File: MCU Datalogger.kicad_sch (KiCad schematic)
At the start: 25 parts, among them U1 24LC1025, U2 DS1337S_, U3 24LC1025, U4 ATMEGA328P-AU, Y1 32.768 KHz, Y2 16 MHz

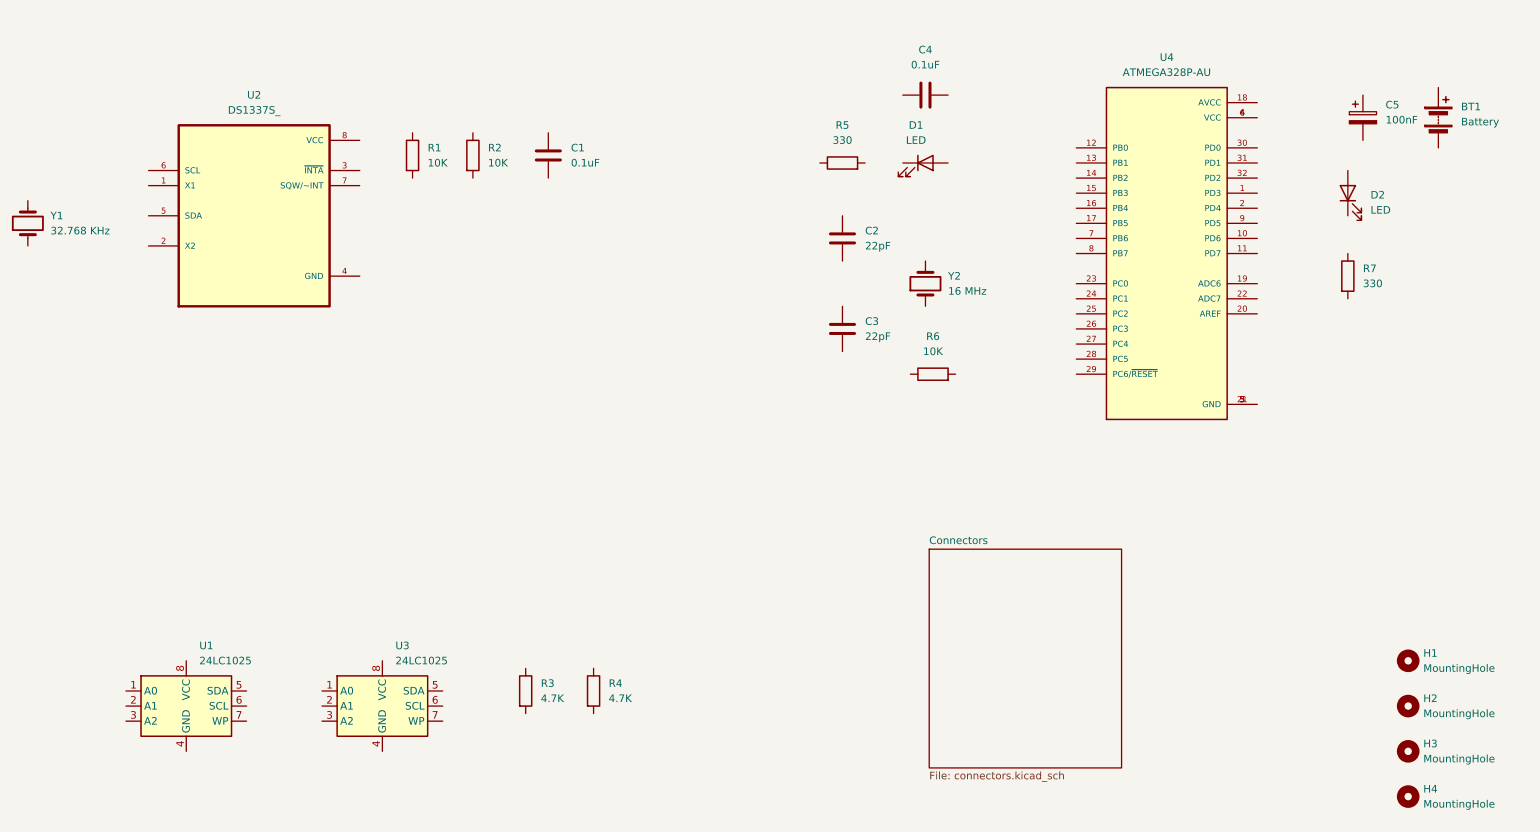
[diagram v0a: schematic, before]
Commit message: Test.
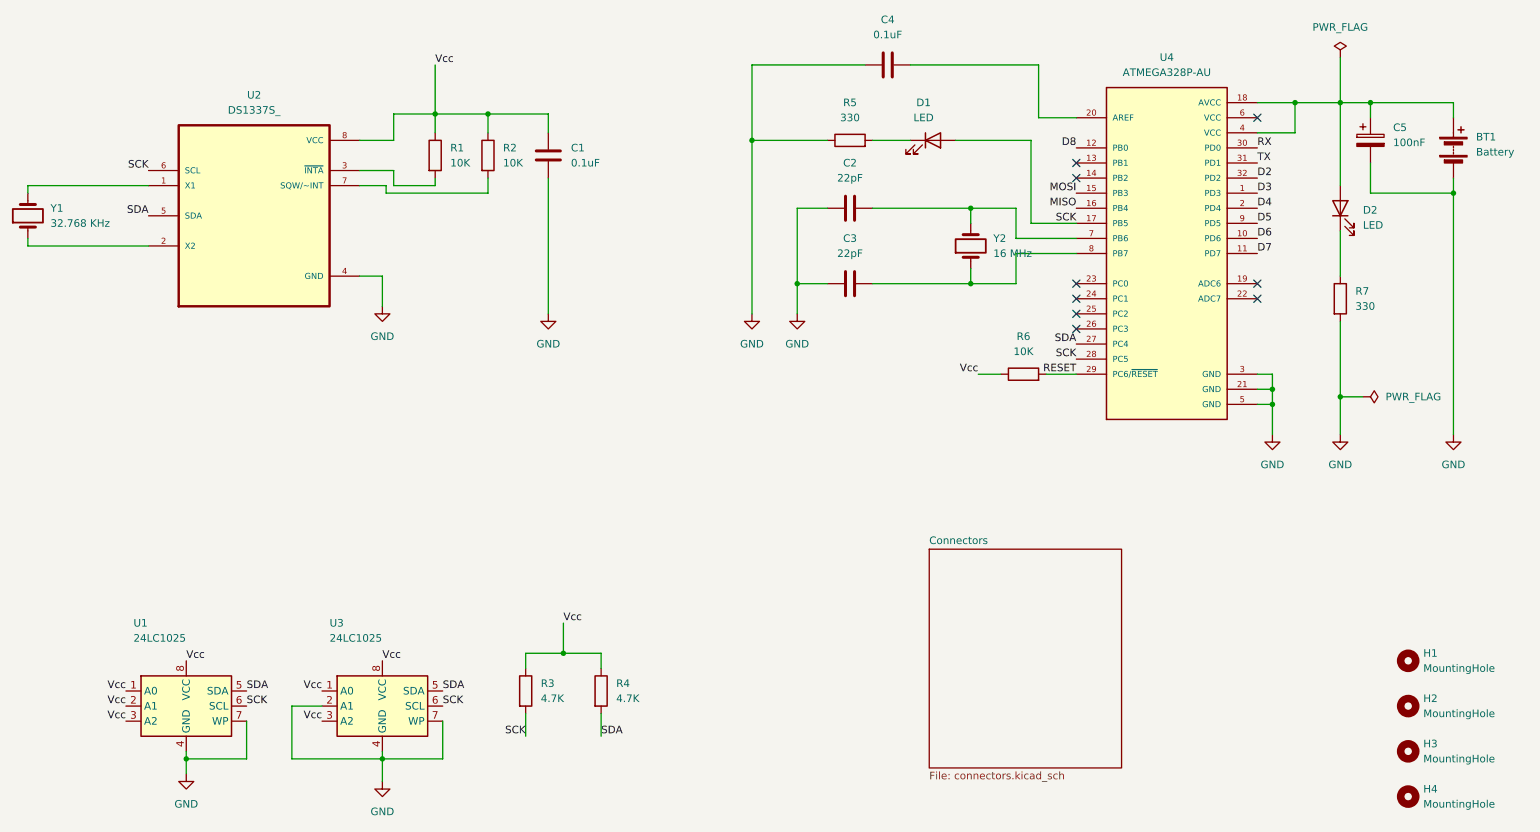
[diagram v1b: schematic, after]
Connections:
- net at Y1.1: now also U2.2 (X2)
- net at Y1.2: now also U2.1 (X1)
- net at C5.1: now also BT1.1 (+), D2.2 (A), U4.18 (AVCC), U4.4 (VCC)
- net GND: now reaches C5.2
- net GND: now also BT1.2 (-), C1.2, C2.1, C3.1, C4.1, R5.1, R7.2, U1.4 (GND), U1.7 (WP), U2.4 (GND), U3.2 (A1), U3.4 (GND), U3.7 (WP), U4.21 (GND), U4.3 (GND), U4.5 (GND)
- net Vcc: now reaches R1.1
- net Vcc: now also C1.1, R2.1, R3.1, R4.1, R6.1, U1.1 (A0), U1.2 (A1), U1.3 (A2), U1.8 (VCC), U2.8 (VCC), U3.1 (A0), U3.3 (A2), U3.8 (VCC)
- net at R1.2: now also U2.3 (~{INTA})
- net at R7.1: now also D2.1 (K)
- net RESET: now reaches R6.2
- net RESET: now also U4.29 (PC6/~{RESET})
- net at C3.2: now also U4.8 (PB7), Y2.1
- net at C2.2: now also U4.7 (PB6), Y2.2
- net SDA: now reaches U2.5 (SDA)
- net SDA: now also R4.2, U1.5 (SDA), U3.5 (SDA), U4.27 (PC4)
- net SCK: now reaches U2.6 (SCL)
- net SCK: now also D1.2 (A), R3.2, U1.6 (SCL), U3.6 (SCL), U4.17 (PB5), U4.28 (PC5)
- net at U2.7 (SQW/~INT): now also R2.2
- net at C4.2: now also U4.20 (AREF)
- net D3: now reaches U4.1 (PD3)
- net D6: now reaches U4.10 (PD6)
- net D7: now reaches U4.11 (PD7)
- net D8: now reaches U4.12 (PB0)
- net MOSI: now reaches U4.15 (PB3)
- net MISO: now reaches U4.16 (PB4)
- net D4: now reaches U4.2 (PD4)
- net RX: now reaches U4.30 (PD0)
- net TX: now reaches U4.31 (PD1)
- net D2: now reaches U4.32 (PD2)
- net at U4.6 (VCC): no longer U4.4 (VCC)
- net D5: now reaches U4.9 (PD5)
- net at R5.2: now also D1.1 (K)
- no-connect marks 0 -> 9
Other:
- moved on the sheet: BT1, C2, C3, C4, C5, D1, D2, R1, R2, R4, R5, R6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
